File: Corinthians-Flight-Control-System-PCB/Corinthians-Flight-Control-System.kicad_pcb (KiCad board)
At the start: 4 copper layers, 48.9 x 72.5 mm, 83 parts, among them J0 RaspberryPi, J1 50ohm Coaxial Ant, J10 M8, J11 M9, J12 M10, J2 GPS/Compass, J3 M1, J4 M2, J5 M3, J6 M4, J7 M5, J8 M6, J9 M7, SW1 BootSW, SW2 SW_DIP_x01, SW3 SW_s, U1 STM32F103C8Tx, U2 LSM6DS3, U3 BMP280, U4 NRF24L01, U5 IST8310, U6 AMS1117-3.3, U7 AMS1117-5.0, Y1 8Mhz, Y2 16Mhz

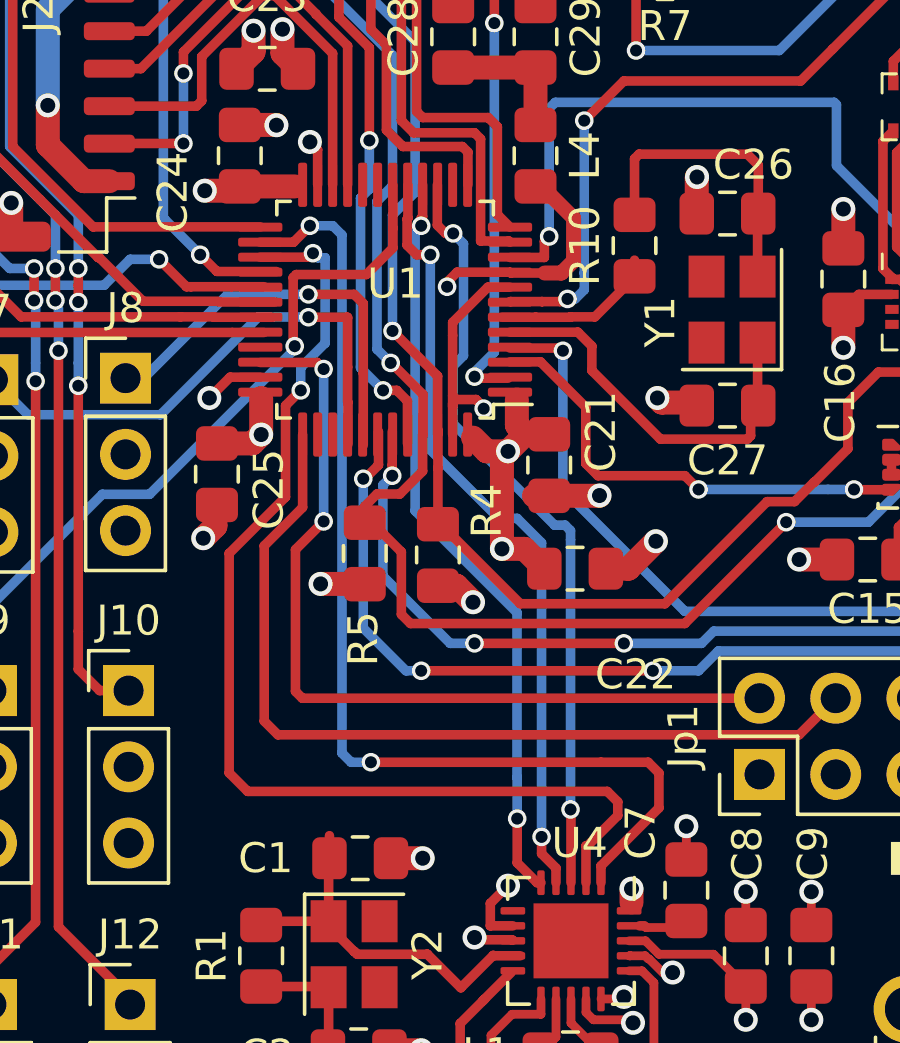
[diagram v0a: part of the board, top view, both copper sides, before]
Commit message: clean
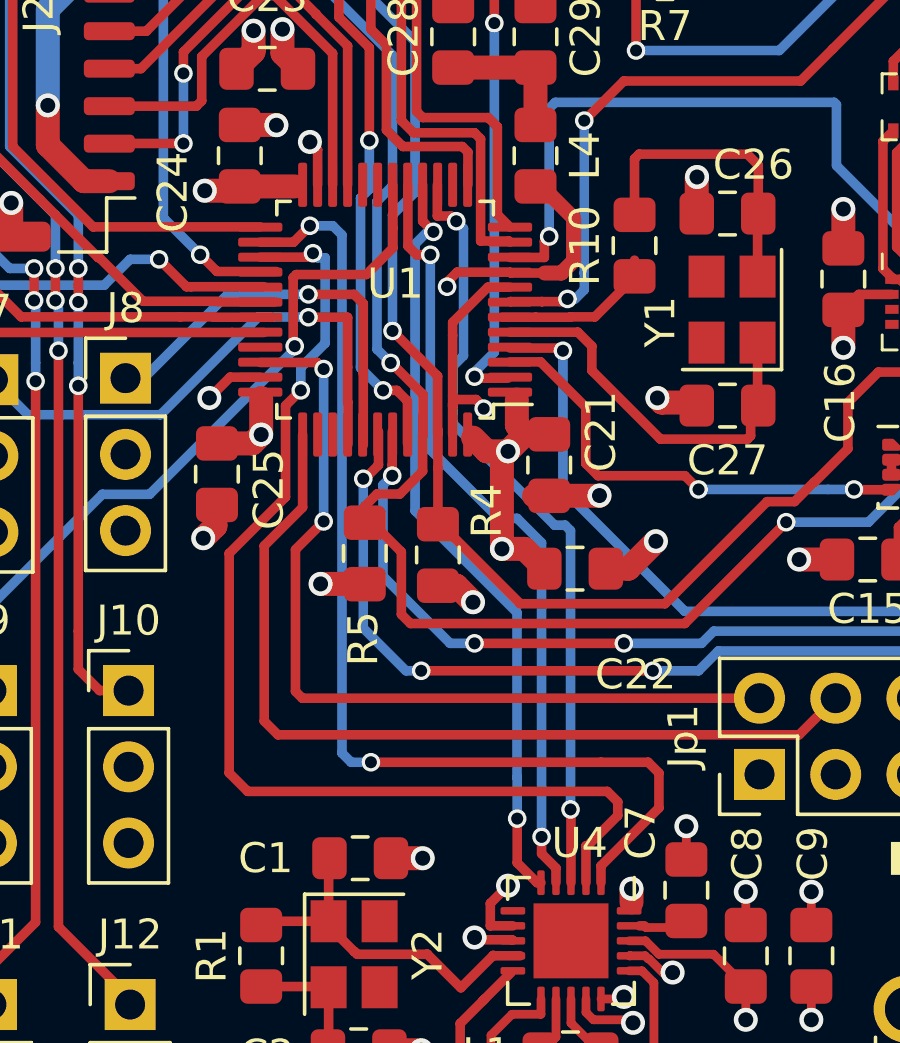
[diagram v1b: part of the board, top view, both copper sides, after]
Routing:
- net Net-(C1-Pad2): track 13.0 -> 12.3 mm
